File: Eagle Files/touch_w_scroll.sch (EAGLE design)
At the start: 8 parts

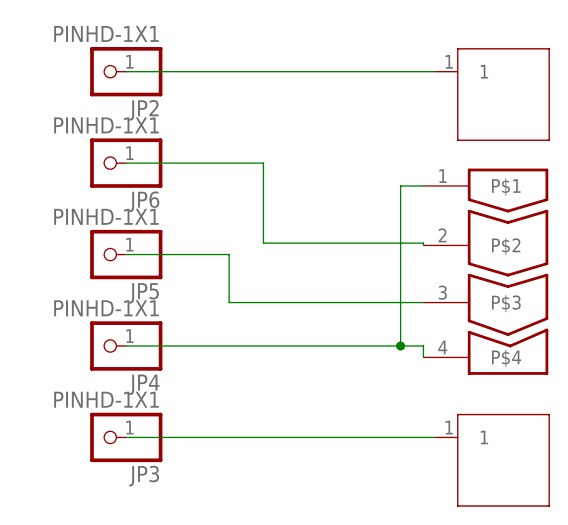
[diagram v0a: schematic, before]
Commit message: updates
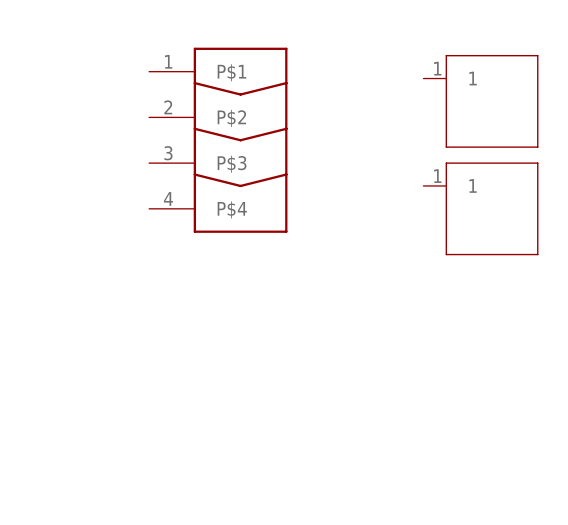
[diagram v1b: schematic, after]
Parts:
- removed JP2, JP3, JP4, JP5, JP6: PINHD-1X1, Connector:PINHD-1X1
- removed U$3: 12X12_PAD, Cap Touch Pads:12X12_PAD
- added U$4: 12X12_PADLED, Cap Touch Pads:12X12_PADLED
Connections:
- removed net N$1: JP3.1, U$3.1
- removed net N$2: JP4.1, U$1.P$1, U$1.P$4
- removed net N$3: JP5.1, U$1.P$3
- removed net N$4: JP6.1, U$1.P$2
- removed net N$5: JP2.1, U$2.1
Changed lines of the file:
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@@
 </classes>
 <parts>
-<part name="U$1" library="Cap Touch Pads" library_urn="urn:adsk.eagle:library:35100943" deviceset="SLIDE_PAD" device="" package3d_urn="urn:adsk.eagle:package:35100947/2"/>
-<part name="U$2" library="Cap Touch Pads" library_urn="urn:adsk.eagle:library:35100943" deviceset="12X12_PAD" device="" package3d_urn="urn:adsk.eagle:package:35100948/1"/>
-<part name="U$3" library="Cap Touch Pads" library_urn="urn:adsk.eagle:library:35100943" deviceset="12X12_PAD" device="" package3d_urn="urn:adsk.eagle:package:35100948/1"/>
-<part name="JP2" library="Connector" library_urn="urn:adsk.eagle:library:16378166" deviceset="PINHD-1X1" device="" package3d_urn="urn:adsk.eagle:package:22485/2"/>
-<part name="JP3" library="Connector" library_urn="urn:adsk.eagle:library:16378166" deviceset="PINHD-1X1" device="" package3d_urn="urn:adsk.eagle:package:22485/2"/>
-<part name="JP4" library="Connector" library_urn="urn:adsk.eagle:library:16378166" deviceset="PINHD-1X1" device="" package3d_urn="urn:adsk.eagle:package:22485/2"/>
-<part name="JP5" library="Connector" library_urn="urn:adsk.eagle:library:16378166" deviceset="PINHD-1X1" device="" package3d_urn="urn:adsk.eagle:package:22485/2"/>
-<part name="JP6" library="Connector" library_urn="urn:adsk.eagle:library:16378166" deviceset="PINHD-1X1" device="" package3d_urn="urn:adsk.eagle:package:22485/2"/>
+<part name="U$1" library="Cap Touch Pads" library_urn="urn:adsk.eagle:library:35100943" deviceset="SLIDE_PAD" device="" package3d_urn="urn:adsk.eagle:package:35100947/4"/>
+<part name="U$2" library="Cap Touch Pads" library_urn="urn:adsk.eagle:library:35100943" deviceset="12X12_PAD" device="" package3d_urn="urn:adsk.eagle:package:35100948/2"/>
+<part name="U$4" library="Cap Touch Pads" library_urn="urn:adsk.eagle:library:35100943" deviceset="12X12_PAD" device="LED" package3d_urn="urn:adsk.eagle:package:35129608/1"/>
 </parts>
 <sheets>
@@
 </plain>
 <instances>
-<instance part="U$1" gate="G$1" x="58.42" y="66.04" smashed="yes"/>
-<instance part="U$2" gate="G$1" x="64.77" y="76.2" smashed="yes"/>
-<instance part="U$3" gate="G$1" x="64.77" y="35.56" smashed="yes"/>
-<instance part="JP2" gate="G$1" x="20.32" y="78.74" smashed="yes" rot="R180">
-<attribute name="NAME" x="26.67" y="75.565" size="1.778" layer="95" rot="R180"/>
-<attribute name="VALUE" x="26.67" y="83.82" size="1.778" layer="96" rot="R180"/>
-</instance>
-<instance part="JP3" gate="G$1" x="20.32" y="38.1" smashed="yes" rot="R180">
-<attribute name="NAME" x="26.67" y="34.925" size="1.778" layer="95" rot="R180"/>
-<attribute name="VALUE" x="26.67" y="43.18" size="1.778" layer="96" rot="R180"/>
-</instance>
-<instance part="JP4" gate="G$1" x="20.32" y="48.26" smashed="yes" rot="R180">
-<attribute name="NAME" x="26.67" y="45.085" size="1.778" layer="95" rot="R180"/>
-<attribute name="VALUE" x="26.67" y="53.34" size="1.778" layer="96" rot="R180"/>
-</instance>
-<instance part="JP5" gate="G$1" x="20.32" y="58.42" smashed="yes" rot="R180">
-<attribute name="NAME" x="26.67" y="55.245" size="1.778" layer="95" rot="R180"/>
-<attribute name="VALUE" x="26.67" y="63.5" size="1.778" layer="96" rot="R180"/>
-</instance>
-<instance part="JP6" gate="G$1" x="20.32" y="68.58" smashed="yes" rot="R180">
-<attribute name="NAME" x="26.67" y="65.405" size="1.778" layer="95" rot="R180"/>
-<attribute name="VALUE" x="26.67" y="73.66" size="1.778" layer="96" rot="R180"/>
-</instance>
+<instance part="U$1" gate="G$1" x="27.94" y="78.74" smashed="yes"/>
+<instance part="U$2" gate="G$1" x="63.5" y="75.438" smashed="yes"/>
+<instance part="U$4" gate="G$1" x="63.5" y="63.5" smashed="yes"/>
 </instances>
 <busses>
 </busses>
 <nets>
-<net name="N$1" class="0">
-<segment>
-<pinref part="U$3" gate="G$1" pin="1"/>
-<wire x1="57.15" y1="38.1" x2="22.86" y2="38.1" width="0.1524" layer="91"/>
-<pinref part="JP3" gate="G$1" pin="1"/>
-</segment>
-</net>
-<net name="N$5" class="0">
-<segment>
-<pinref part="U$2" gate="G$1" pin="1"/>
-<wire x1="22.86" y1="78.74" x2="57.15" y2="78.74" width="0.1524" layer="91"/>
-<pinref part="JP2" gate="G$1" pin="1"/>
-</segment>
-</net>
-<net name="N$2" class="0">
-<segment>
-<pinref part="JP4" gate="G$1" pin="1"/>
-<pinref part="U$1" gate="G$1" pin="P$4"/>
-<wire x1="22.86" y1="48.26" x2="53.34" y2="48.26" width="0.1524" layer="91"/>
-<wire x1="53.34" y1="48.26" x2="55.88" y2="48.26" width="0.1524" layer="91"/>
-<wire x1="55.88" y1="48.26" x2="55.88" y2="46.99" width="0.1524" layer="91"/>
-<pinref part="U$1" gate="G$1" pin="P$1"/>
-<wire x1="53.34" y1="48.26" x2="53.34" y2="66.04" width="0.1524" layer="91"/>
-<wire x1="53.34" y1="66.04" x2="55.88" y2="66.04" width="0.1524" layer="91"/>
-<junction x="53.34" y="48.26"/>
-</segment>
-</net>
-<net name="N$3" class="0">
-<segment>
-<pinref part="U$1" gate="G$1" pin="P$3"/>
-<wire x1="55.88" y1="53.086" x2="34.29" y2="53.086" width="0.1524" layer="91"/>
-<wire x1="34.29" y1="53.086" x2="34.29" y2="58.42" width="0.1524" layer="91"/>
-<pinref part="JP5" gate="G$1" pin="1"/>
-<wire x1="34.29" y1="58.42" x2="22.86" y2="58.42" width="0.1524" layer="91"/>
-</segment>
-</net>
-<net name="N$4" class="0">
-<segment>
-<pinref part="U$1" gate="G$1" pin="P$2"/>
-<wire x1="55.88" y1="59.436" x2="55.88" y2="59.69" width="0.1524" layer="91"/>
-<wire x1="55.88" y1="59.69" x2="38.1" y2="59.69" width="0.1524" layer="91"/>
-<wire x1="38.1" y1="59.69" x2="38.1" y2="68.58" width="0.1524" layer="91"/>
-<pinref part="JP6" gate="G$1" pin="1"/>
-<wire x1="38.1" y1="68.58" x2="22.86" y2="68.58" width="0.1524" layer="91"/>
-</segment>
-</net>
 </nets>
 </sheet>
